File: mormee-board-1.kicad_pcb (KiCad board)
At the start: 4 copper layers, 201 x 119.5 mm, 160 parts, among them J1 PDM MEMS Mic, J2 24FLZ-SM2-TB, J3 USB4105-GF-A, J4 Conn_01x02, J5 DM3BT-DSF-PEJS, Q1 AO3401A, SW1 EVQ-PUB02K, SW2 EVQ-PUB02K, U1 W25Q128JVSIQ, U10 MAX17048G+T10, U11 MP2637GR-P, U2 RTL8735BDM-A20-N04, U3 FDS9926A, U4 FT232RNL-REEL, U5 RT8097AHGE, U6 RT8097AHGE, U7 RT9080-28GJ5, U8 RT9080-18GJ5, U9 RT9080-12GJ5

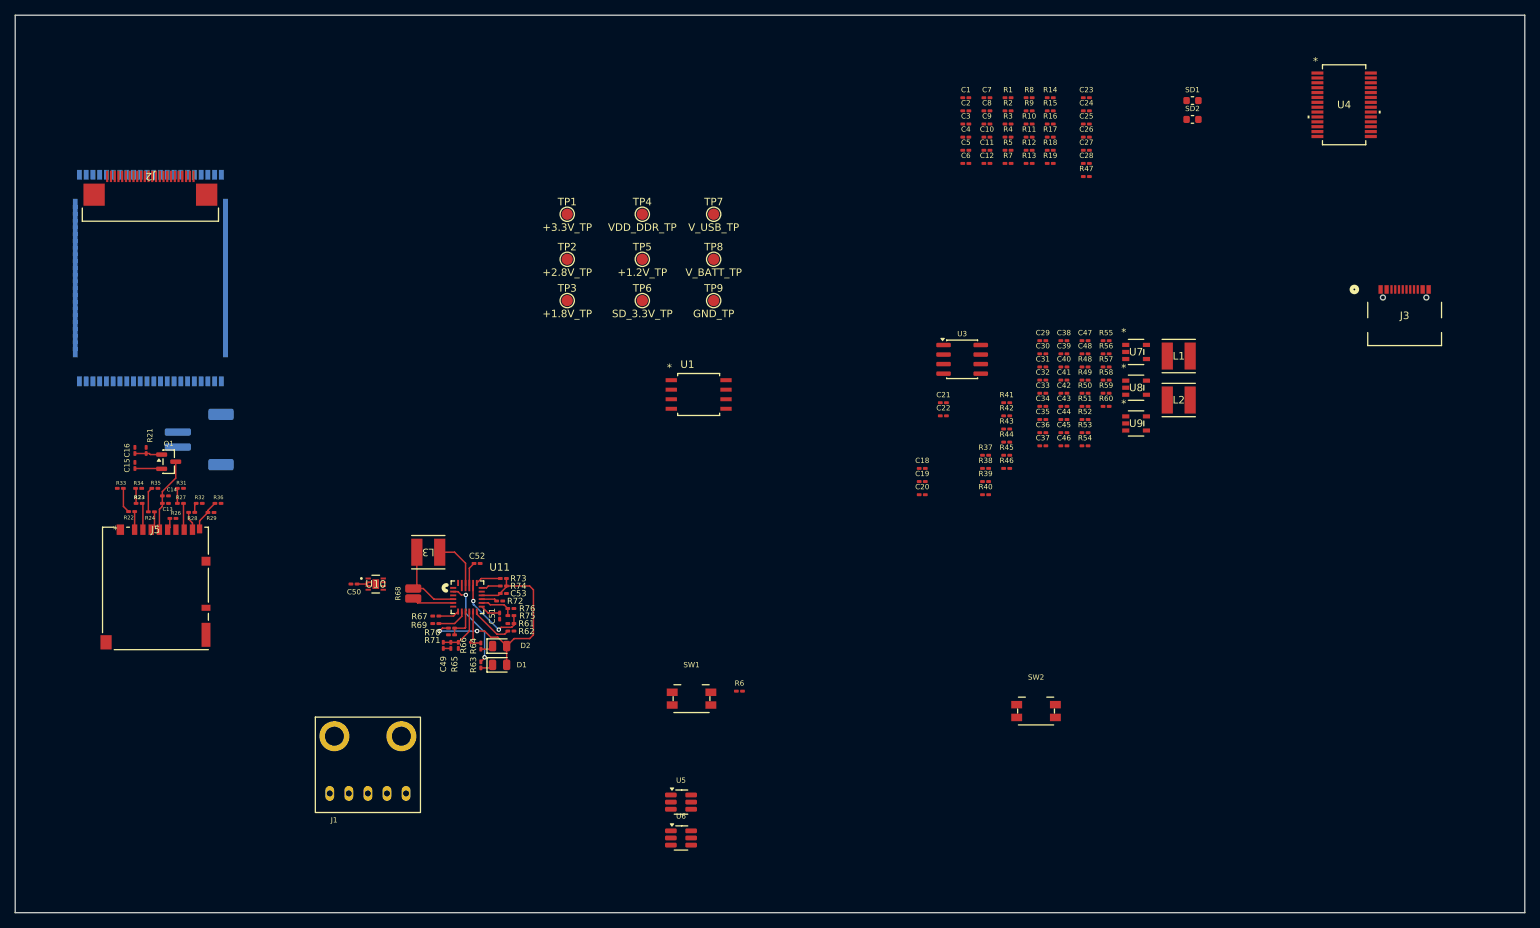
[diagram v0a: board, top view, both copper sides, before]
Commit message: Breakthrough in PCB layout. WIP
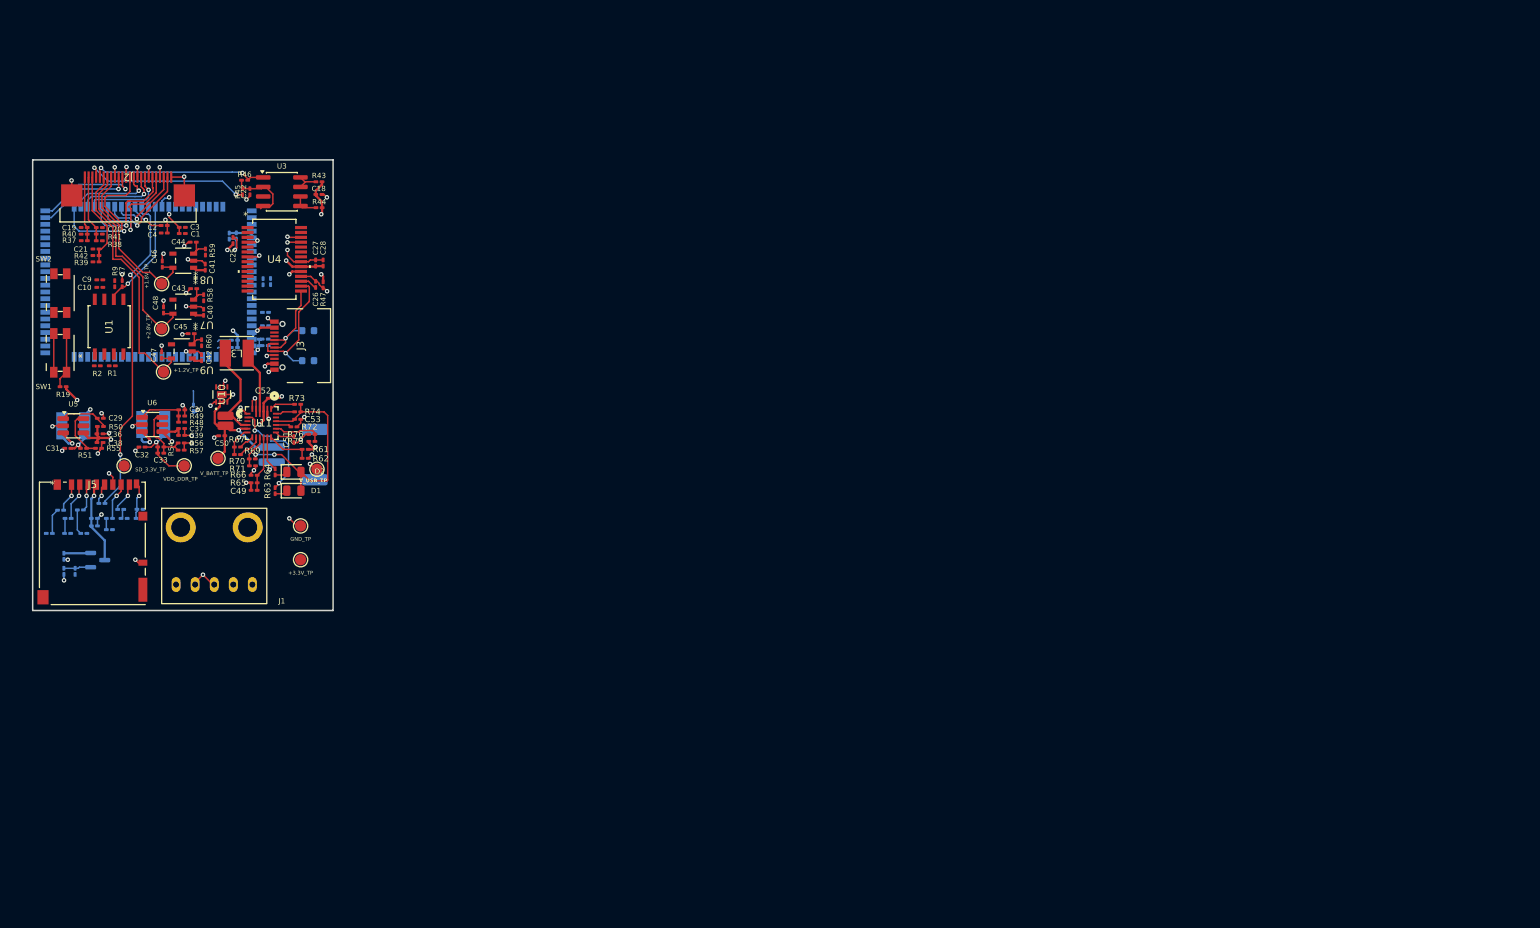
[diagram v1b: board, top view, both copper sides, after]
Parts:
- removed C34, C35: 10uF, Capacitor_SMD:C_0201_0603Metric_Pad0.64x0.40mm_HandSolder
- removed R10, R11, R18, R3, R4, R5, R52, R53, R6, R7, R8: 0, Resistor_SMD:R_0201_0603Metric_Pad0.64x0.40mm_HandSolder
- C11, C12, C13, C14, C15, C16, C23, C24, C5, C6, C8, L1, L2, Q1, R12, R13, R14, R15, R16, R17, R21, R22, R23, R24, R26, R27, R28, R29, R31, R32, R33, R34, R35, R36, SD1, SD2: moved to B.Cu
- moved L1 147.5 mm to (74.7, 76.2), turned to 180 degrees
- moved J3 147.1 mm to (105.0, 65.5), turned to 90 degrees
- moved U4 143.9 mm to (101.5, 54.0)
- moved SW2 141.3 mm to (73.0, 58.5), turned to 90 degrees
- moved L2 136.6 mm to (85.4, 76.0), turned to 180 degrees
- moved R55 134.9 mm to (78.1, 79.2)
- moved R19 134.8 mm to (73.4, 71.0), turned to 180 degrees
- moved R51 133.5 mm to (76.1, 79.2)
- moved R50 131.2 mm to (78.3, 76.3)
- moved C31 130.3 mm to (74.0, 79.2), turned to 180 degrees
- moved C38 129.1 mm to (78.3, 78.4)
- moved U8 128.0 mm to (89.4, 54.2), turned to 180 degrees
- moved U9 127.4 mm to (89.2, 66.3), turned to 180 degrees
- moved U7 127.0 mm to (89.4, 60.3), turned to 180 degrees
- moved R2 125.9 mm to (77.9, 68.2), turned to 180 degrees
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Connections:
- net Net-(U11-CSP) renamed /Battery/L3
- net Net-(U11-SW) renamed /Battery/SW
- net Net-(U5-LX) renamed /Power/L1
- net Net-(U6-LX) renamed /Power/L2
- C10 pad 1: SOC_FLASH -> +3.3V
- C31 pad 1: Net-(C31-Pad1) -> +3.3V
- C32 pad 1: Net-(C32-Pad1) -> VDD_DDR
- C33 pad 2: Net-(C32-Pad1) -> VDD_DDR
- C9 pad 1: SOC_FLASH -> +3.3V
- J1 pad 4: /SD CARD /Vidio / Audio / USB/DMIC_CLK -> DMIC_CLK
- J1 pad 5: /SD CARD /Vidio / Audio / USB/DMIC_DATA -> DMIC_DATA
- L1 pad 1: Net-(C31-Pad1) -> +3.3V
- L2 pad 1: Net-(C32-Pad1) -> VDD_DDR
- R1 pad 1: SOC_FLASH -> +3.3V
- R12 pad 2: /RTL9835B/LOG_IN -> CH_UART_TX
- R13 pad 2: /RTL9835B/LOG_OUT -> CH_UART_RX
- R2 pad 1: SOC_FLASH -> +3.3V
- R51 pad 1: Net-(C31-Pad1) -> +3.3V
- R54 pad 1: Net-(C32-Pad1) -> VDD_DDR
- R9 pad 1: SOC_FLASH -> +3.3V
- U1 pad 8: SOC_FLASH -> +3.3V
- U2 pad 1: Net-(U2-FLASH_D3) -> /RTL9835B/FLASH_D3
- U2 pad 2: Net-(U2-FLASH_D1) -> /RTL9835B/FLASH_D1
- U2 pad 31: /RTL9835B/DMIC_CLK -> DMIC_CLK
- U2 pad 35: /RTL9835B/DMIC_DATA -> DMIC_DATA
- U2 pad 48: Net-(U2-UART1_IN) -> CH_UART_TX
- U2 pad 49: Net-(U2-UART1_OUT) -> CH_UART_RX
- U2 pad 77: Net-(U2-MIC1_P) -> /RTL9835B/MIC1_P
- U2 pad 88: Net-(U2-FLASH_D0) -> /RTL9835B/FLASH_D0
- U2 pad 89: Net-(U2-FLASH_D2) -> /RTL9835B/FLASH_D2
- U2 pad 90: Net-(U2-FLASH_CS) -> /RTL9835B/FLASH_CS
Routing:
- net GND: track 0.00 -> 103.7 mm, vias 0 -> 61
- net SD_CLK: track 0.00 -> 43.1 mm, vias 0 -> 2
- net SEN_1V2: track 0.00 -> 34.8 mm
- net +3.3V: track 3.58 -> 37.9 mm, vias 0 -> 9
- net SEN_1V8: track 0.00 -> 31.7 mm
- net SEN_2V8: track 0.00 -> 28.5 mm
- net /SD CARD /Vidio / Audio / USB/SDA: track 0.00 -> 23.5 mm, vias 0 -> 2
- net /SD CARD /Vidio / Audio / USB/SCL: track 0.00 -> 22.5 mm, vias 0 -> 2
- net MDN2: track 0.00 -> 20.6 mm, vias 0 -> 1
- net /Debug Interface/USB_N: track 0.00 -> 18.1 mm, vias 0 -> 1
- net VDD_DDR: track 0.00 -> 16.8 mm, vias 0 -> 2
- net MDP1: track 0.00 -> 15.5 mm, vias 0 -> 1
- net /RTL9835B/FLASH_CLK: track 0.00 -> 14.8 mm, vias 0 -> 1
- net MDN1: track 0.00 -> 14.8 mm, vias 0 -> 1
- net MDP3: track 0.00 -> 14.1 mm, vias 0 -> 1
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- added copper zone on In2.Cu, net +3.3V
- added copper zone on In2.Cu, net +5V
- added copper zone on In1.Cu, net GND
- added copper zone on In2.Cu, net V_USB
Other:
- board size 201 x 119.5 mm -> 40 x 60 mm
